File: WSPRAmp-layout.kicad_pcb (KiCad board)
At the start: 2 copper layers, 101 x 64 mm, 22 parts, among them J1 Conn_Coaxial_Small, J2 Conn_01x05, U3 T2N7002AK_G0_00

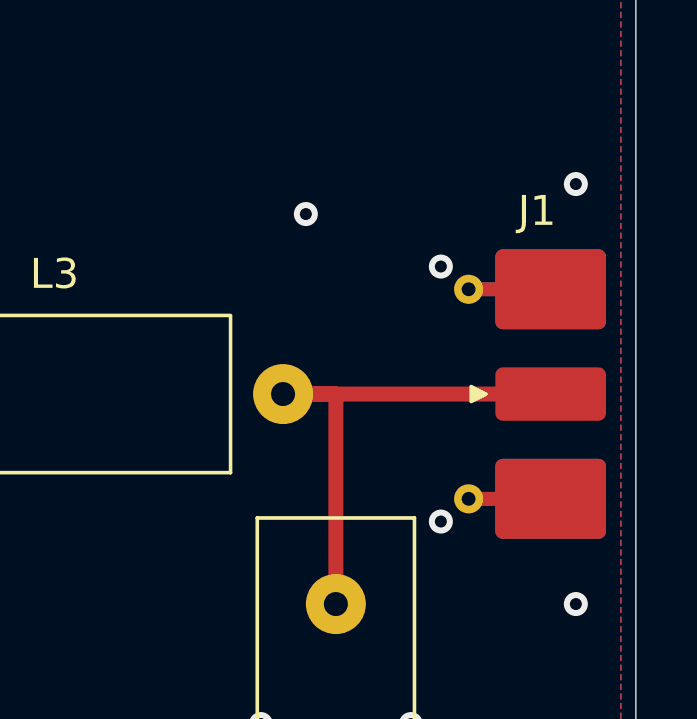
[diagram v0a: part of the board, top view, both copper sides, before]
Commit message: Sumbit to DKRed, etc
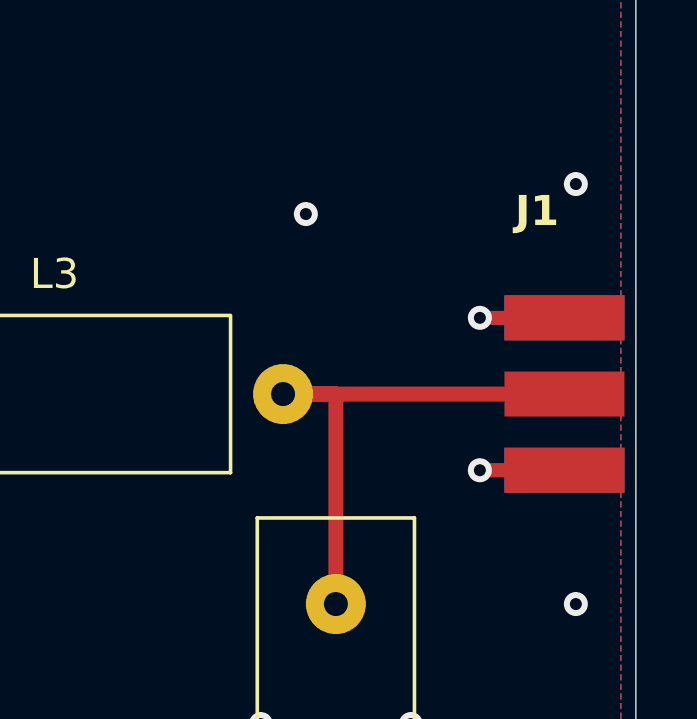
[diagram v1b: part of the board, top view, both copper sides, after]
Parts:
- J1: footprint Connector_Coaxial:SMA_Molex_73251-2120_EdgeMount_Horizontal -> WSPRAmp:SMA_Edge_6.3mm
- moved J1 0.21 mm to (138.6, 53.0), turned to -90 degrees
